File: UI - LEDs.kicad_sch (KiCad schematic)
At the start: 2 parts

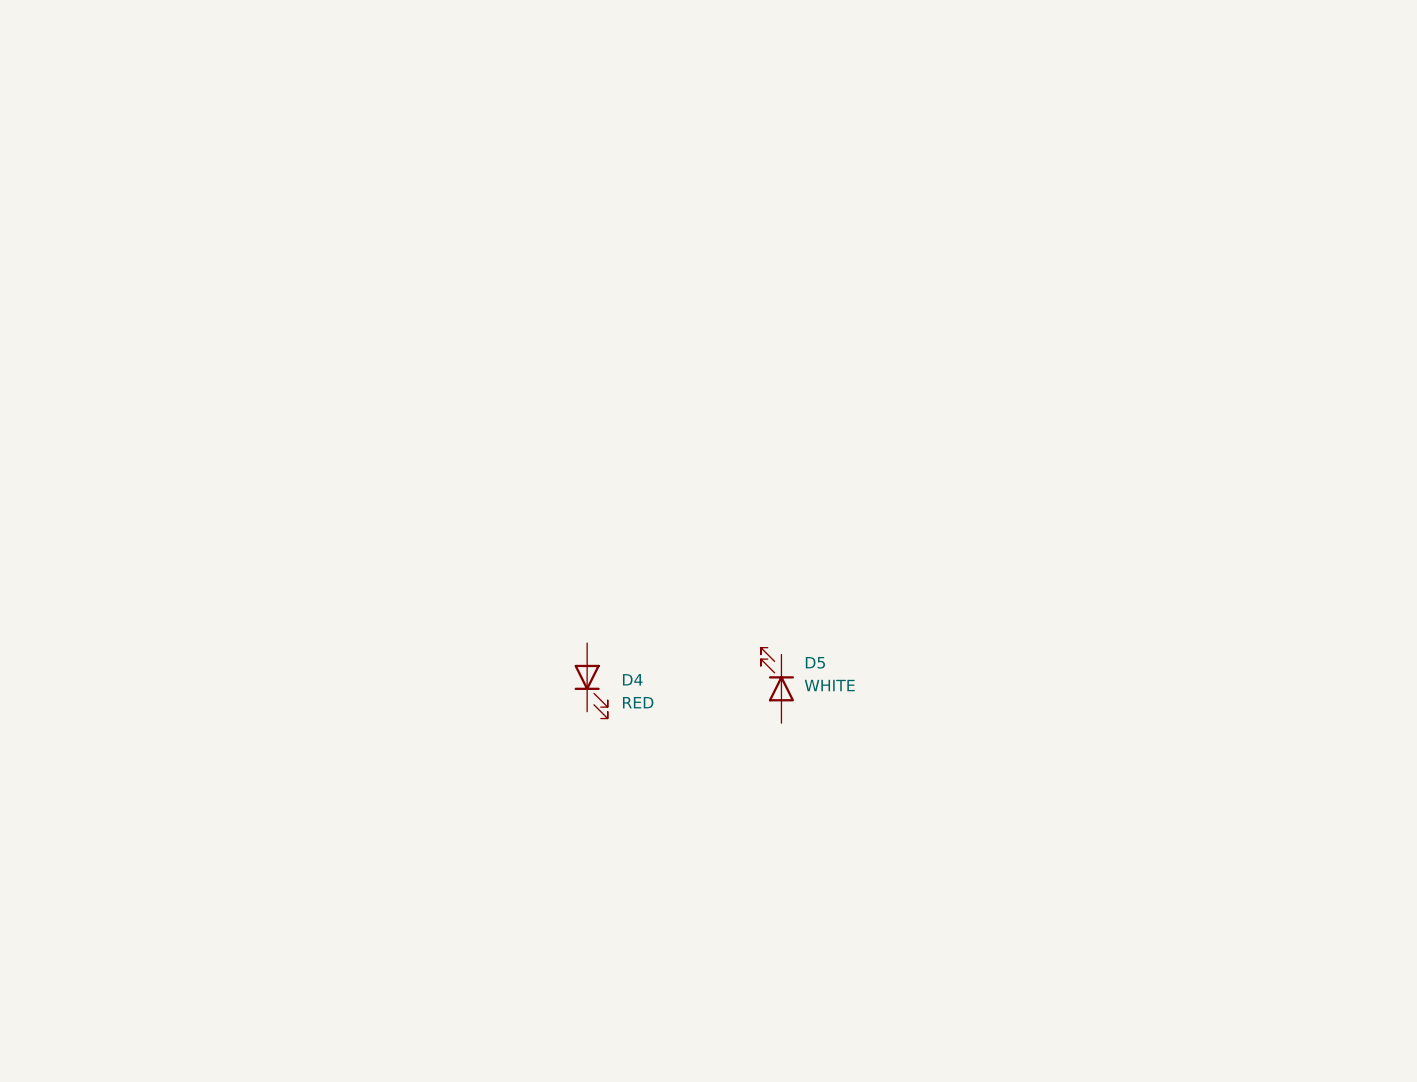
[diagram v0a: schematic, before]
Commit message: led schematic
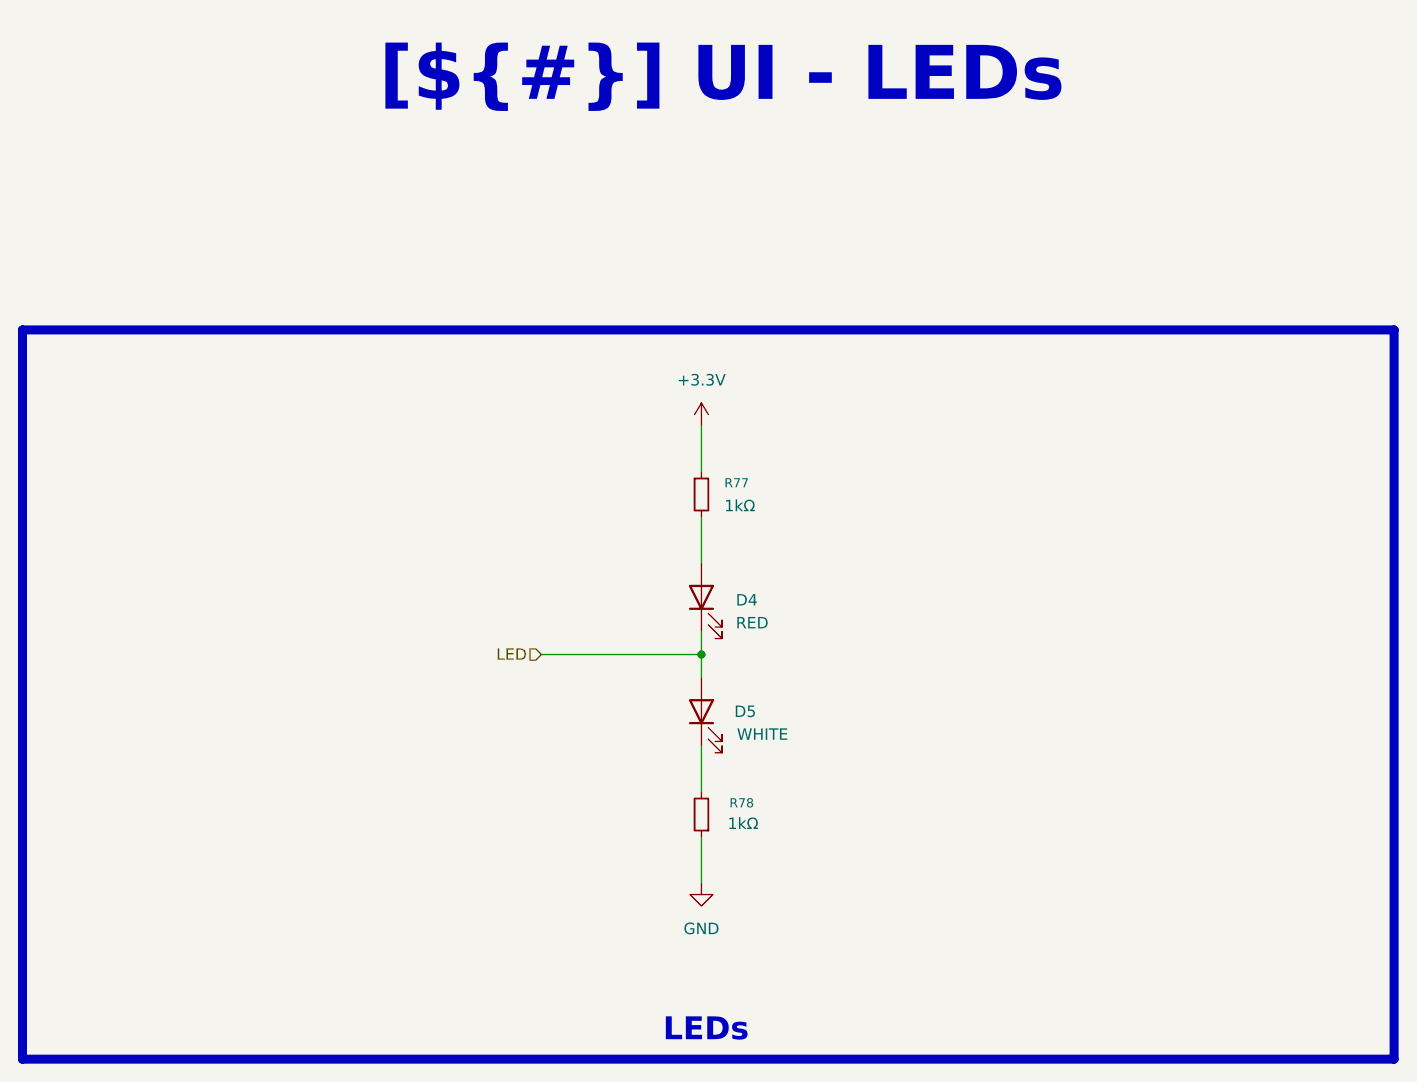
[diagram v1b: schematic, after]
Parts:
- added R77, R78: 1kΩ, 0_resistors:R_0402_1005Metric, symbol 0_resistors:0402WGF1001TCE
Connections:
- net at D5.1 (K): now also R78.2
- net LED: now reaches D5.2 (A)
- net LED: now also D4.1 (K)
- net at D4.2 (A): now also R77.2
- new net +3.3V: R77.1
- new net GND: R78.1
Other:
- moved on the sheet: D4, D5

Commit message: designator chagnes and cleanup silkscreen
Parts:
- D4: LCSC PN (none) -> 0603
- D5: LCSC PN (none) -> C2290
- R77, R78: LCSC PN (none) -> C11702
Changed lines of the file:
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@@
+			)
+		)
+		(property "LCSC PN" "C11702"
+			(at 146.05 101.6 0)
+			(effects
+				(font
+					(size 1.27 1.27)
+				)
+				(hide yes)
 			)
 		)
@@
 			)
 		)
+		(property "LCSC PN" "C2290"
+			(at 146.05 90.17 0)
+			(effects
+				(font
+					(size 1.27 1.27)
+				)
+				(hide yes)
+			)
+		)
 		(pin "1"
 		)
@@
 			)
 		)
+		(property "LCSC PN" "0603"
+			(at 146.05 77.47 0)
+			(effects
+				(font
+					(size 1.27 1.27)
+				)
+				(hide yes)
+			)
+		)
 		(pin "2"
 		)
@@
 			(at 146.05 66.04 0)
 			(effects
+				(font
+					(size 1.27 1.27)
+				)
+				(hide yes)
+			)
+		)
+		(property "LCSC PN" "C11702"
+			(at 146.05 66.04 0)
+			(effects
